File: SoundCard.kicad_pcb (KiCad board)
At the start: 2 copper layers, 20.3 x 51.6 mm, 38 parts, among them J1 Conn_Coaxial_inv, J2 Conn_01x03_Female, J3 Conn_01x03_Female, P1 CONN_36_P1.00_PCI, U1 LM334M, U2 LM1972, U3 OPA2388IDGK, U4 OPA1692xD

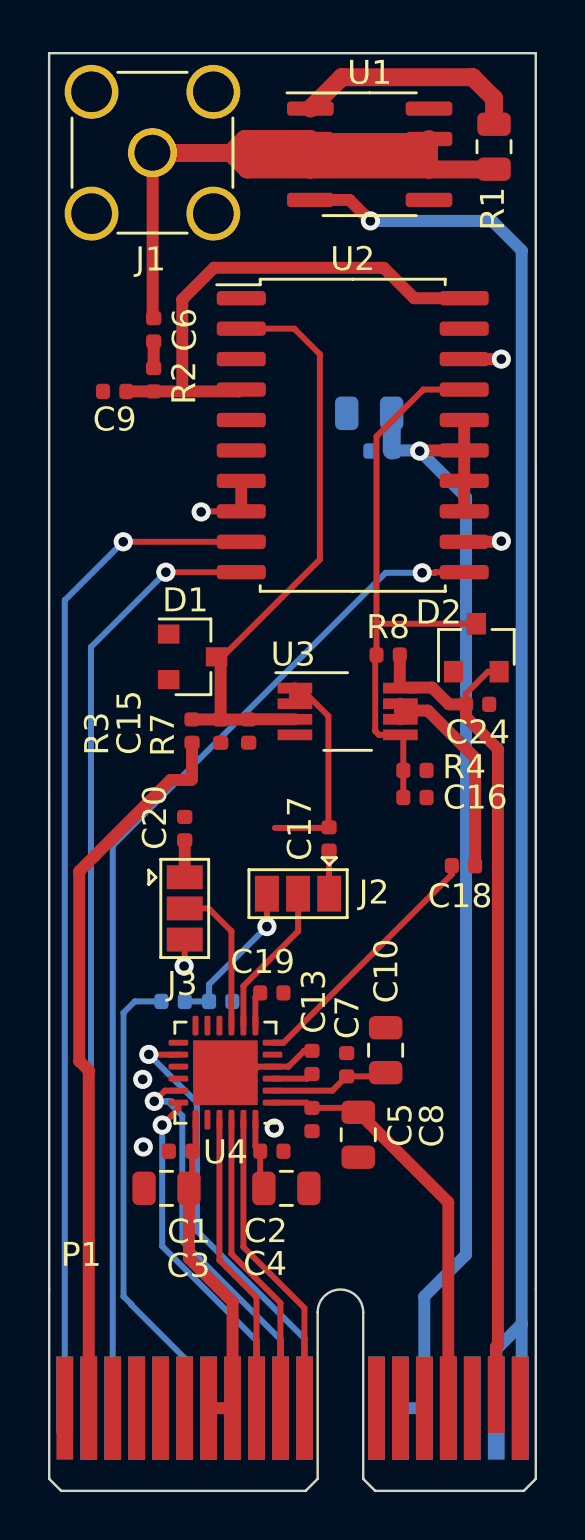
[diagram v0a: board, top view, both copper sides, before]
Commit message: routage terminé
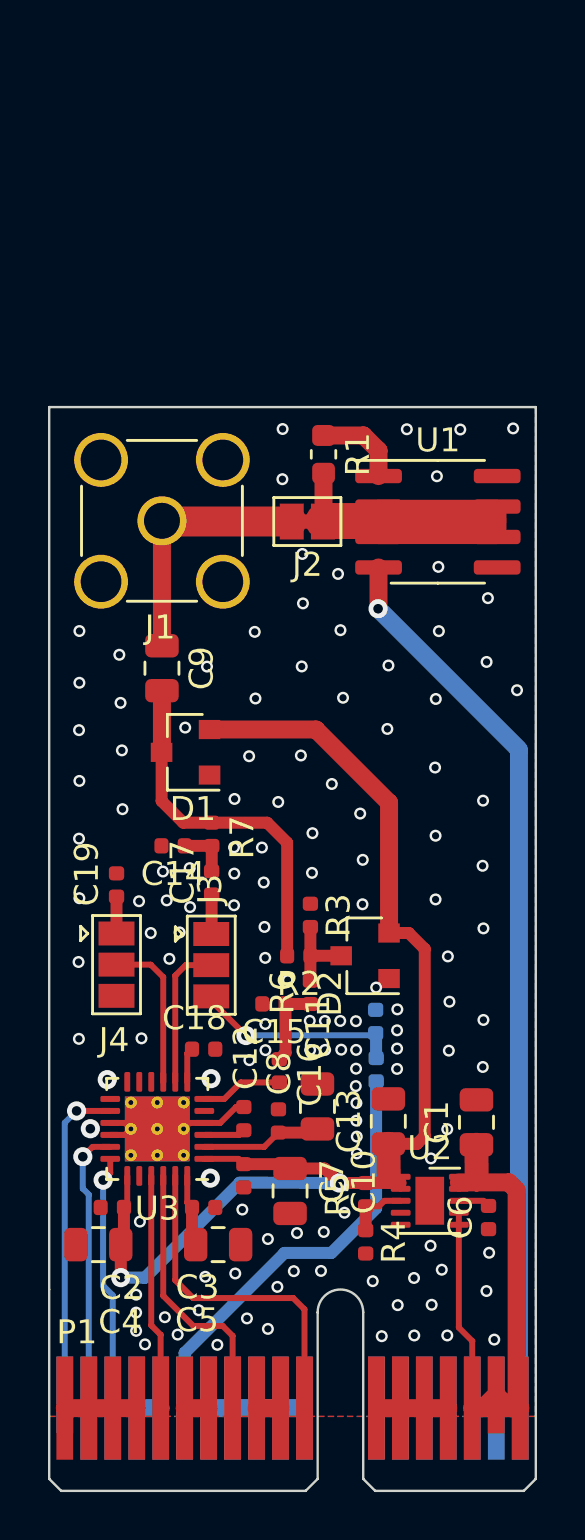
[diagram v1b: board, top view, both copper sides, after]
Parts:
- removed the C16 at (148.1, 124.9)
- removed C22, C24: 0.1uF, Capacitor_SMD:C_0402_1005Metric
- removed C23: 10uF, Capacitor_SMD:C_0805_2012Metric
- removed the R8 at (146.9, 118.9)
- removed the U3 at (145.3, 121.3)
- added C1: 10uF, Capacitor_SMD:C_0805_2012Metric, F.Cu at (150.6, 138.4)
- added C13: 10uF, Capacitor_SMD:C_0805_2012Metric, F.Cu at (146.9, 138.4)
- added C6: 1uF, Capacitor_SMD:C_0402_1005Metric, F.Cu at (151.1, 142.4)
- added J2: Conn_01x02_Female, Jumper:SolderJumper-2_P1.3mm_Bridged_Pad1.0x1.5mm, F.Cu at (143.6, 113.4)
- added R5: 3.57k, Resistor_SMD:R_0402_1005Metric, F.Cu at (146.0, 141.5)
- added R6: 33.2, Resistor_SMD:R_0402_1005Metric, F.Cu at (143.7, 133.0)
- C14: renamed from C9; value 8pF -> 200nF
- C15: value 1uF -> 200nF
- C9: renamed from C6; value 1uF -> 4.7uF; footprint Capacitor_SMD:C_0402_1005Metric -> Capacitor_SMD:C_0805_2012Metric
- R1: footprint Resistor_SMD:R_0805_2012Metric -> Resistor_SMD:R_0603_1608Metric
- R3: value 10k -> 750
- R4: value 10k -> 1.15k
- R7: value 10k -> 33.2
- U2: value LM1972 -> TPS7A90; footprint Package_SO:SOIC-20W_7.5x12.8mm_P1.27mm -> Package_DFN_QFN:Texas_S-PDSO-N10_EP1.2x2mm
- U3: renamed from U4; value OPA1692xD -> TLV320ADC6140; footprint Package_DFN_QFN:Texas_S-PWQFN-N24_EP2.7x2.7mm -> Package_DFN_QFN:Texas_S-PWQFN-N24_EP2.7x2.7mm_ThermalVias
- moved U2 32.1 mm to (148.7, 141.7)
- moved R2 24.8 mm to (143.2, 131.5), turned to 180 degrees
- moved R4 19.8 mm to (146.0, 143.4), turned to 270 degrees
- moved C14 19.1 mm to (138.0, 126.9)
- moved U1 15.6 mm to (149.0, 113.4)
- moved J1 15.4 mm to (137.5, 113.4)
- moved R1 14.7 mm to (144.2, 110.6)
- moved C9 14.1 mm to (137.5, 119.5)
- moved D2 13.7 mm to (146.0, 131.5), turned to 180 degrees
- moved C16 11.5 mm to (142.4, 136.3), turned to 270 degrees
- moved C15 11.4 mm to (142.2, 133.5), turned to 180 degrees
- moved R9 8.94 mm to (146.4, 136.2), turned to 270 degrees
- moved R3 8.55 mm to (143.7, 129.8), turned to 270 degrees
- moved R8 6.52 mm to (146.4, 134.2), turned to 270 degrees
- moved C17 5.23 mm to (139.6, 128.5)
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- renumbered C8 to C10, C10 to C11, C13 to C12, C18 to C16, C19 to C18, C20 to C19, C1 to C2, C2 to C3, C3 to C4, C4 to C5, C5 to C7, C7 to C8, J2 to J3, J3 to J4, R9 to R8, R10 to R9
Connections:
- C10 pad 1: VDDA -> VDD
- C10 pad 2: GNDA -> GND
- C11 pad 2: GNDA -> GND
- C12 pad 1: GNDA -> GND
- C14 pad 1: /CH1_IEPE_OUT -> Net-(C14-Pad1)
- C14 pad 2: GNDA -> GND
- C15 pad 1: GNDA -> Net-(C15-Pad1)
- C15 pad 2: /ATT_OUT1 -> GND
- C16 pad 1: Net-(C18-Pad1) -> Net-(C15-Pad1)
- C17 pad 1: Net-(C17-Pad1) -> Net-(C14-Pad1)
- C17 pad 2: (no net) -> /ENHANCE_CH1
- C18 pad 2: GNDA -> GND
- C19 pad 2: GNDA -> GND
- C2 pad 1: GNDD -> GND
- C3 pad 1: GNDD -> GND
- C4 pad 2: GNDD -> GND
- C5 pad 2: GNDD -> GND
- C7 pad 1: GNDA -> GND
- C7 pad 2: VDDA -> VDD
- C8 pad 1: GNDA -> GND
- C9 pad 1: Net-(C6-Pad1) -> Net-(C9-Pad1)
- C9 pad 2: Net-(C6-Pad2) -> /IEPE_OUT
- D1 pad 1: GNDA -> GND
- D1 pad 2: VDDA -> VDD
- D1 pad 3: /ATT_OUT1 -> /IEPE_OUT
- D2 pad 1: GNDA -> GND
- D2 pad 2: VDDA -> VDD
- D2 pad 3: /ATT_OUT2 -> /IEPE_OUT_ATT
- J1 pad 1: Net-(C6-Pad1) -> Net-(C9-Pad1)
- J1 pad 2: GNDA -> GND
- J3 pad 1: (no net) -> /ENHANCE_CH1
- J4 pad 3: GNDD -> GND
- P1 pad A1: /ATT_CLOCK -> /SHDNZ
- P1 pad A10: /SCL -> GND
- P1 pad A11: /SHDNZ -> GND
- P1 pad A12: (no net) -> GND
- P1 pad A13: VCC -> GND
- P1 pad A14: VCC -> GND
- P1 pad A15: GNDD -> GND
- P1 pad A16: GNDD -> +24V
- P1 pad A2: /ATT_~CS~ -> /SCL
- P1 pad A3: /ATT_DATA_IN -> /SDA
- P1 pad A4: (no net) -> GND
- P1 pad A5: (no net) -> GND
- P1 pad A7: (no net) -> GND
- P1 pad A8: (no net) -> GND
- P1 pad A9: /SDA -> GND
- P1 pad B1: GNDA -> GND
- P1 pad B10: /BCLK -> GND
- P1 pad B12: GNDA -> GND
- P1 pad B13: GNDA -> GND
- P1 pad B14: GNDA -> GND
- P1 pad B15: VDDA -> GND
- P1 pad B16: GNDA -> VCC
- P1 pad B17: VDDA -> VCC
- P1 pad B18: GNDA -> VCC
- P1 pad B2: VDDA -> GND
- P1 pad B3: GNDA -> GND
- P1 pad B4: (no net) -> GND
- P1 pad B5: GNDD -> /SDOUT
- P1 pad B6: GNDD -> GND
- P1 pad B7: VDD -> GND
- P1 pad B8: VDD -> /BCLK
- P1 pad B9: /SDOUT -> GND
- R1 pad 2: Net-(C6-Pad1) -> Net-(J2-Pad1)
- R2 pad 1: /CH1_IEPE_OUT -> /IEPE_OUT_ATT
- R2 pad 2: Net-(C6-Pad2) -> /IEPE_OUT
- R3 pad 1: GNDA -> GND
- R3 pad 2: /ATT_OUT1 -> /IEPE_OUT_ATT
- R4 pad 1: GNDA -> Net-(R4-Pad1)
- R4 pad 2: /ATT_OUT2 -> GND
- R7 pad 1: /ATT_OUT1 -> Net-(C14-Pad1)
- R7 pad 2: VDDA -> /IEPE_OUT
- R8 pad 1: GNDD -> GND
- U1 pad 2: Net-(C6-Pad1) -> Net-(J2-Pad1)
- U1 pad 3: Net-(C6-Pad1) -> Net-(J2-Pad1)
- U1 pad 6: Net-(C6-Pad1) -> Net-(J2-Pad1)
- U1 pad 7: Net-(C6-Pad1) -> Net-(J2-Pad1)
- U2 pad 1: GNDA -> VDD
- U2 pad 10: /ATT_~CS~ -> VCC
- U2 pad 11: /ATT_DATA_IN -> GND
- U2 pad 2: /ATT_OUT1 -> VDD
- U2 pad 3: GNDA -> Net-(R4-Pad1)
- U2 pad 4: /CH1_IEPE_OUT -> GND
- U2 pad 5: GNDA -> (no net)
- U2 pad 6: GNDA -> VCC
- U2 pad 7: GNDD -> VCC
- U2 pad 8: GNDD -> Net-(C6-Pad2)
- U2 pad 9: /ATT_CLOCK -> VCC
- U3 pad 1: VDDA -> VDD
- U3 pad 15: GNDD -> GND
- U3 pad 16: GNDD -> GND
- U3 pad 25: GNDA -> GND
- U3 pad 4: GNDA -> GND
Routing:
- net VDDA: track 83.7 -> 0.00 mm
- net Net-(C6-Pad1): track 43.6 -> 0.00 mm
- net /ATT_DATA_IN: track 42.9 -> 0.00 mm, vias 1 -> 0
- net /ATT_CLOCK: track 41.5 -> 0.00 mm, vias 1 -> 0
- net /ATT_~CS~: track 39.4 -> 0.00 mm, vias 1 -> 0
- net VDD: track 13.9 -> 51.0 mm, vias 0 -> 2
- net VCC: track 50.9 -> 24.2 mm, vias 1 -> 0
- net /ATT_OUT1: track 25.0 -> 0.00 mm
- net /ATT_OUT2: track 24.8 -> 0.00 mm
- net +24V: track 62.0 -> 39.5 mm
- net /CH1_IEPE_OUT: track 21.5 -> 0.00 mm
- net Net-(J2-Pad1): track 0.00 -> 19.8 mm
- net GND: track 0.00 -> 18.7 mm, vias 0 -> 135
- net /IEPE_OUT: track 0.00 -> 15.3 mm
- net Net-(C9-Pad1): track 0.00 -> 10.6 mm
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- added copper zone on B.Cu, net GND
- added copper zone on F.Cu, net GND
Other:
- board size 20.3 x 51.6 mm -> 20.3 x 36.8 mm
